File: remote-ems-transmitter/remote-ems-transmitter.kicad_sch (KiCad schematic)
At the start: 57 parts, among them IC1 Wio-E5, J1 Conn_01x04_Pin, J2 Conn_01x02, J3 Conn_01x02, J4 Conn_Coaxial, J5 USB_C_Receptacle_USB2.0, J6 Conn_01x02_Pin, Q1 BSS138, SW1 SW_Push, SW2 SW_Push, SW3 SW_Push, SW4 2MS1-T2-B4-VS2-Q-E-S, U1 STM32G431K8Tx, U2 MCP73831-2-OT, U3 NJM12888F33, U4 XC8111AA01MR-G, U5 XC8111AA01MR-G

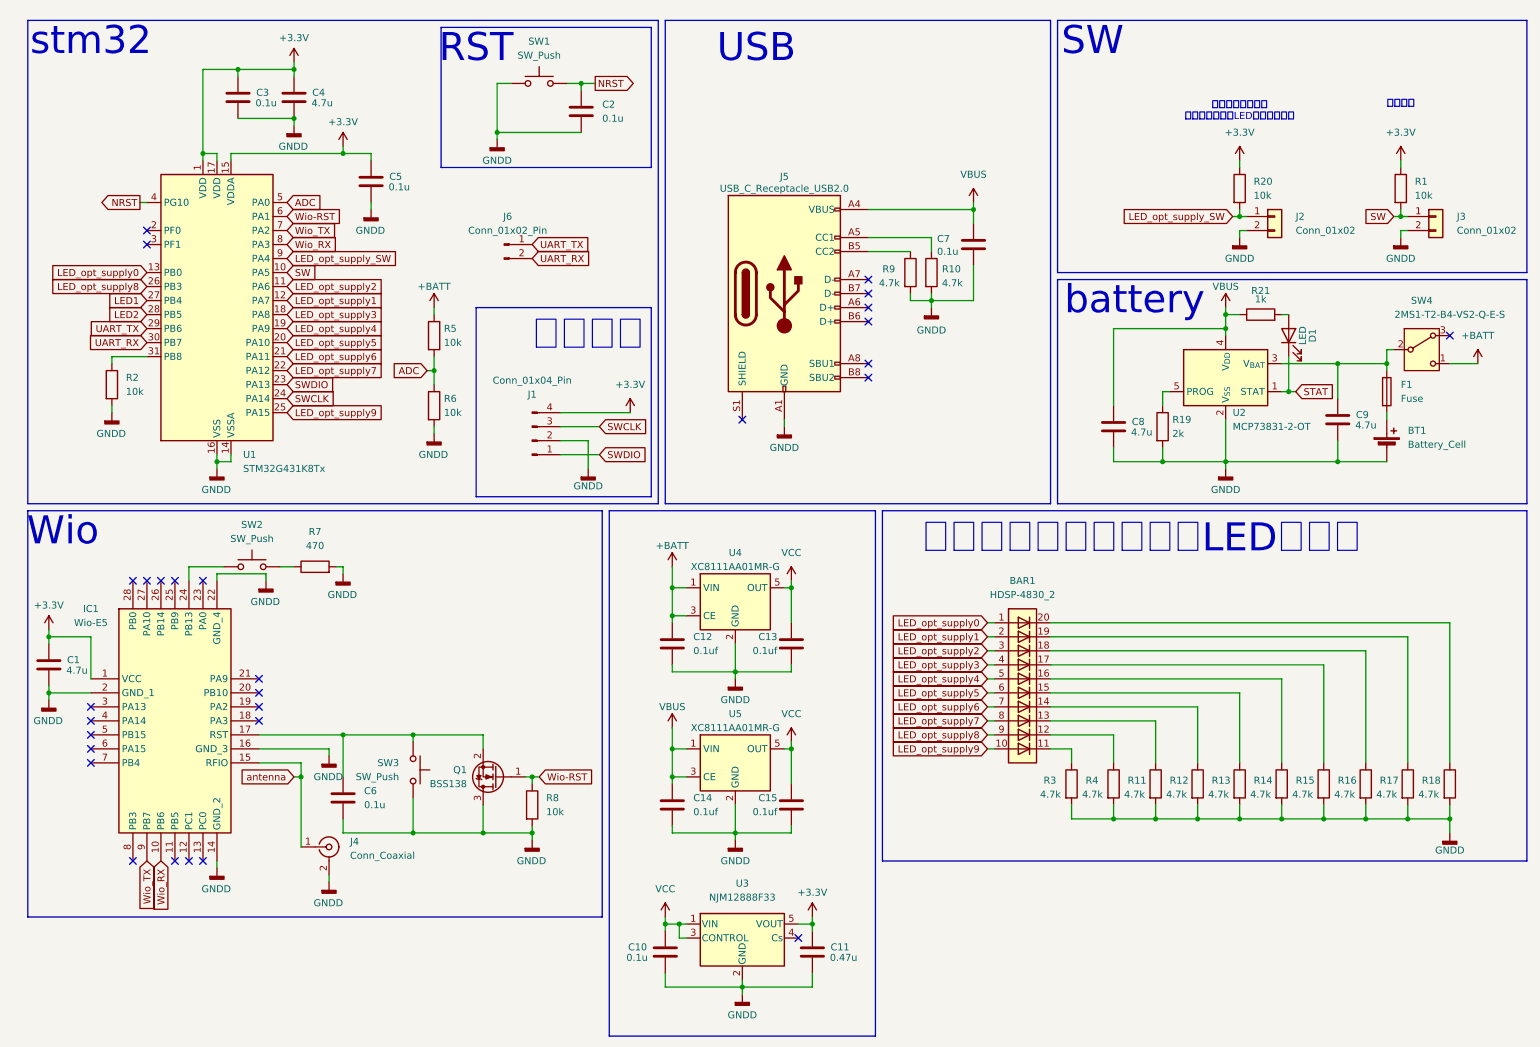
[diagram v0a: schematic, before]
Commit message: LED周り修正
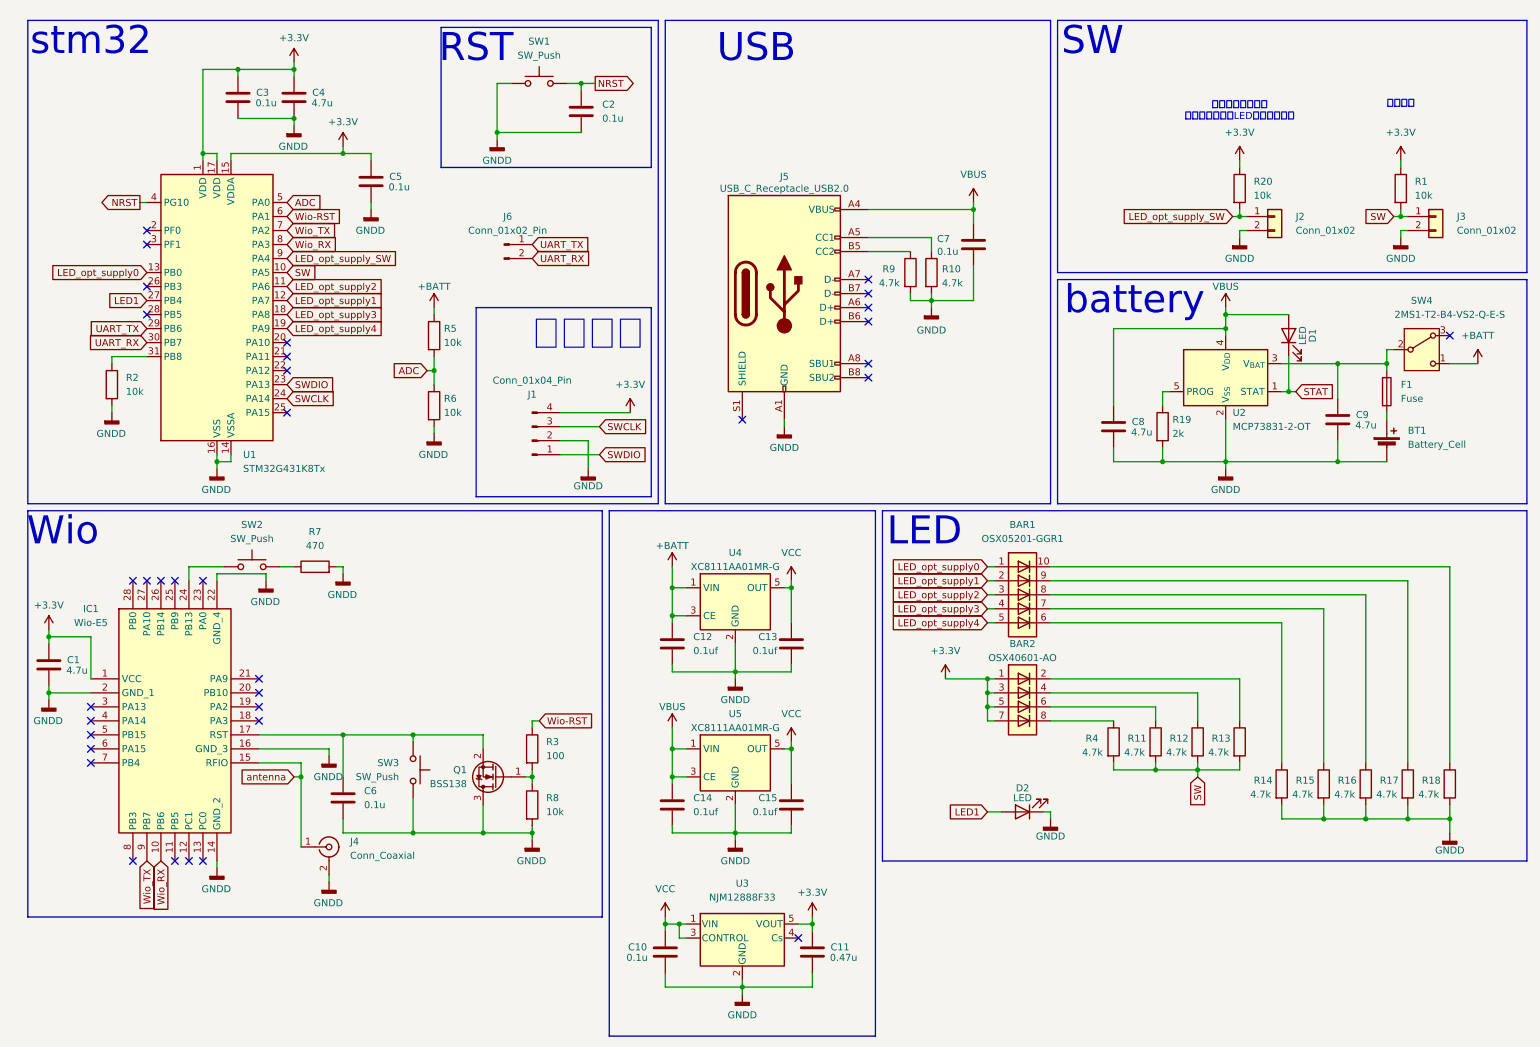
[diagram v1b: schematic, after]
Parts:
- removed R21: 1k, Resistor_SMD:R_0603_1608Metric_Pad0.98x0.95mm_HandSolder, symbol Device:R
- added BAR2: OSX40601-AO, 0Ikedalibrary:OSX40601-AO, symbol LED:HDSP-4830_2
- added D2: LED, LED_THT:LED_D5.0mm_FlatTop, symbol Device:LED
- BAR1: value HDSP-4830_2 -> OSX05201-GGR1; footprint Display:HDSP-4830 -> 0Ikedalibrary:OSX05201-GGR1
- D1: footprint LED_SMD:LED_0603_1608Metric_Pad1.05x0.95mm_HandSolder -> LED_THT:LED_D5.0mm_FlatTop
- R3: value 4.7k -> 100
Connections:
- net +3.3V: now also BAR2.1 (A), BAR2.3 (A), BAR2.5 (A), BAR2.7 (K)
- net GNDD: now also D2.1 (K); no longer R11.2, R12.2, R13.2, R3.2, R4.2
- net LED1: now also D2.2 (A)
- net SW: now also R11.2, R12.2, R13.2, R4.2
- net VBUS: now also D1.2 (A)
- net Wio-RST: now also R3.1; no longer Q1.1 (G), R8.1
- net at R14.1: now also BAR1.6 (K); no longer BAR1.16 (K)
- net at R18.1: now also BAR1.10 (K); no longer BAR1.20 (K)
- net at R4.1: now also BAR2.8 (K); no longer BAR1.12 (K)
- net at R11.1: now also BAR2.6 (K); no longer BAR1.13 (K)
- net at R12.1: now also BAR2.4 (A); no longer BAR1.14 (K)
- net at R13.1: now also BAR2.2 (A); no longer BAR1.15 (K)
- net at R15.1: now also BAR1.7 (K); no longer BAR1.17 (K)
- net at R16.1: now also BAR1.8 (K); no longer BAR1.18 (K)
- net at R17.1: now also BAR1.9 (K); no longer BAR1.19 (K)
- net LED2: no longer names the net of U1.28 (PB5)
- net LED_opt_supply5: no longer names the net of U1.20 (PA10)
- net LED_opt_supply5: no longer BAR1.6 (A)
- net LED_opt_supply6: no longer names the net of U1.21 (PA11)
- net LED_opt_supply6: no longer BAR1.7 (A)
- net LED_opt_supply7: no longer names the net of U1.22 (PA12)
- net LED_opt_supply7: no longer BAR1.8 (A)
- net LED_opt_supply8: no longer names the net of U1.26 (PB3)
- net LED_opt_supply8: no longer BAR1.9 (A)
- net LED_opt_supply9: no longer names the net of U1.25 (PA15)
- net LED_opt_supply9: no longer BAR1.10 (A)
- new net: Q1.1 (G), R3.2, R8.1
- no-connect marks 29 -> 35
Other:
- note added: "LED"
- note removed: "バッテリー残量監視用LEDアレイ"
- moved on the sheet: R11, R12, R13, R4

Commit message: LED仕様変更
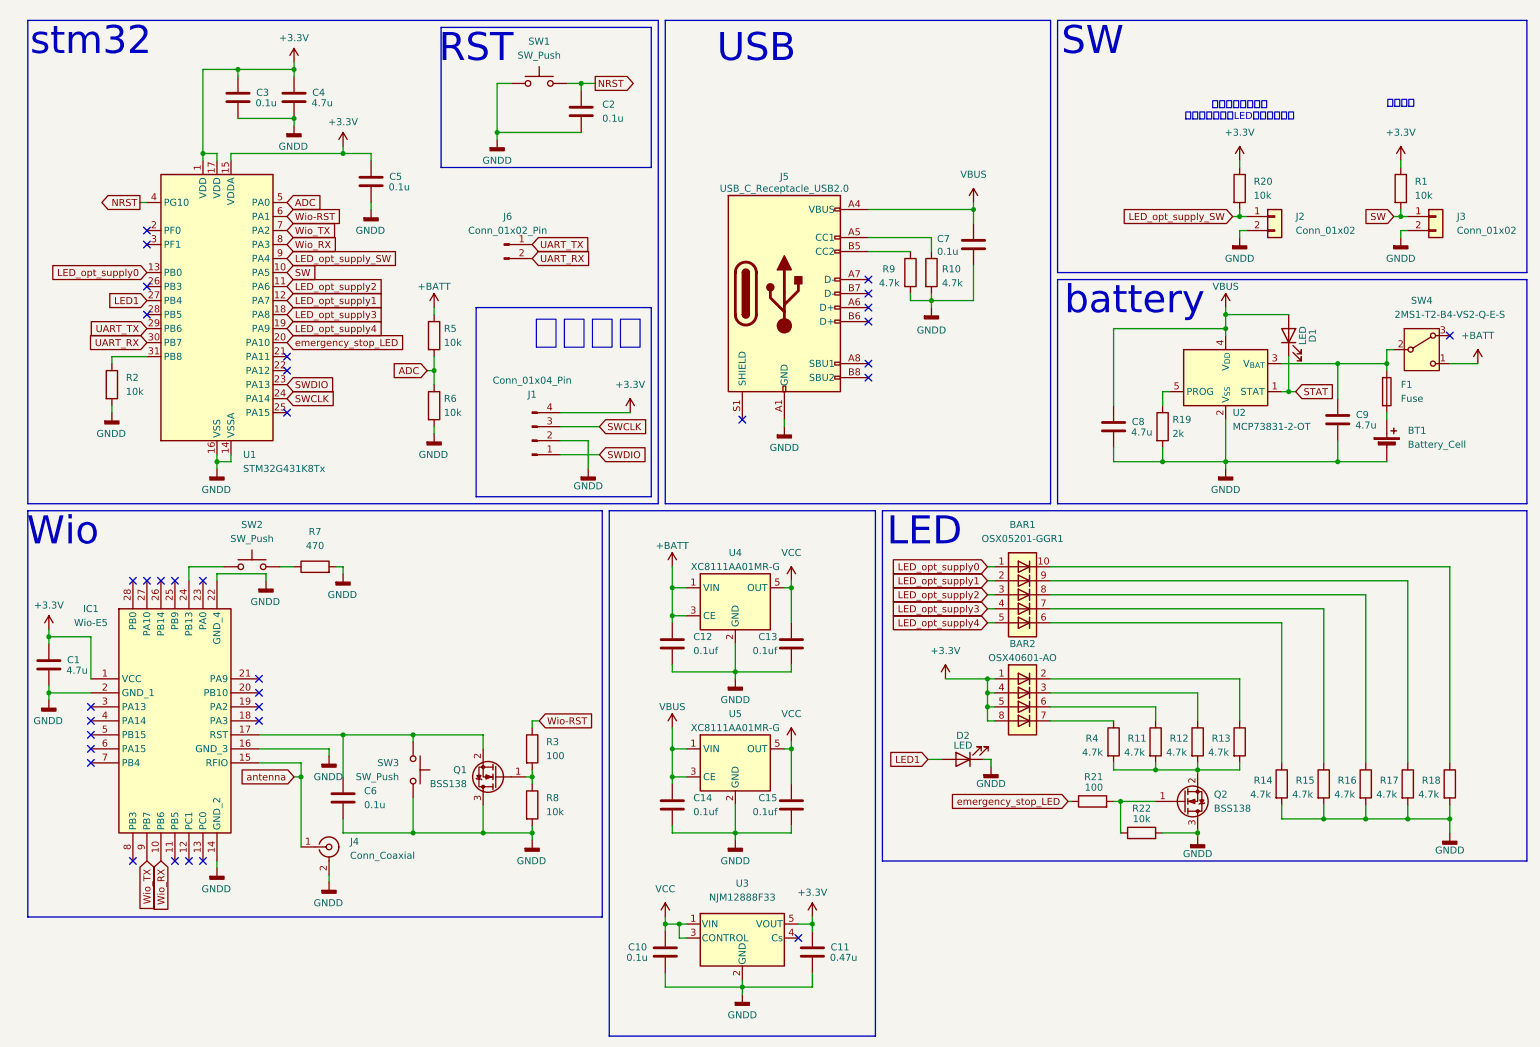
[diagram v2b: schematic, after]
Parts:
- added Q2: BSS138, Package_TO_SOT_SMD:SOT-23, symbol Transistor_FET:BSS138
- added R21: 100, Resistor_SMD:R_0603_1608Metric_Pad0.98x0.95mm_HandSolder, symbol Device:R
- added R22: 10k, Resistor_SMD:R_0603_1608Metric_Pad0.98x0.95mm_HandSolder, symbol Device:R
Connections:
- net +3.3V: now also BAR2.4 (A), BAR2.8 (K); no longer BAR2.3 (A), BAR2.7 (K)
- net GNDD: now also Q2.3 (D), R22.2
- net SW: no longer R11.2, R12.2, R13.2, R4.2
- net at R4.1: now also BAR2.7 (K); no longer BAR2.8 (K)
- net at R12.1: now also BAR2.3 (A); no longer BAR2.4 (A)
- net emergency_stop_LED: now reaches U1.20 (PA10)
- net emergency_stop_LED: now also R21.1
- new net: Q2.1 (G), R21.2, R22.1
- new net: Q2.2 (S), R11.2, R12.2, R13.2, R4.2
- no-connect marks 35 -> 34
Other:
- moved on the sheet: D2
